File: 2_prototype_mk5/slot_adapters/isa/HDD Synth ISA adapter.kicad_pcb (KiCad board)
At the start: 2 copper layers, 119.4 x 97.4 mm, 16 parts, among them J1 Conn_01x02_Socket, J2 Conn_01x05_Socket, J3 Bus_ISA_8bit, J4 Conn_01x02_Socket, SW1 SW_Push, SW2 PEC12R-2120F-S0012

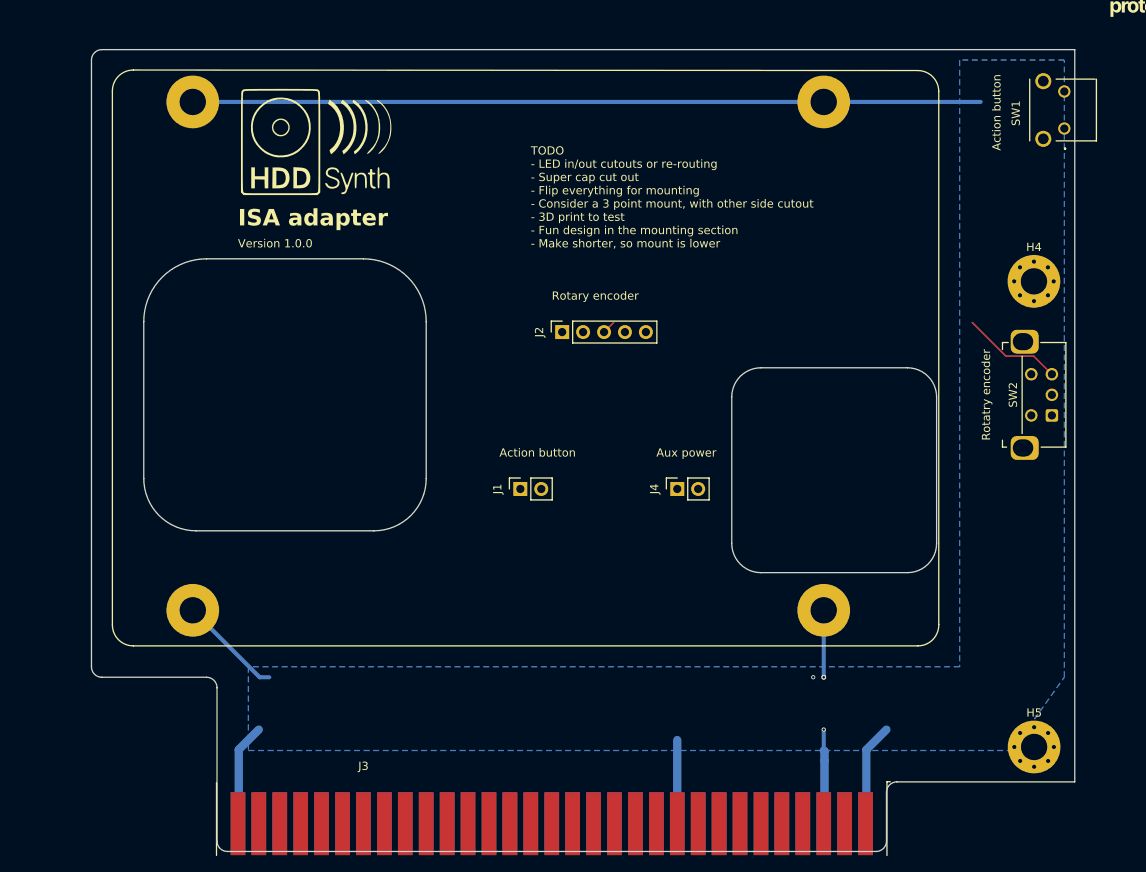
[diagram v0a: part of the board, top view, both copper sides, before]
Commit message: MK5 revision 2 hardware updates and ISA adapter revisions
Ignore VSCode local-history artifacts going forward.

Co-Authored-By: Claude Sonnet 5 <noreply@anthropic.com>
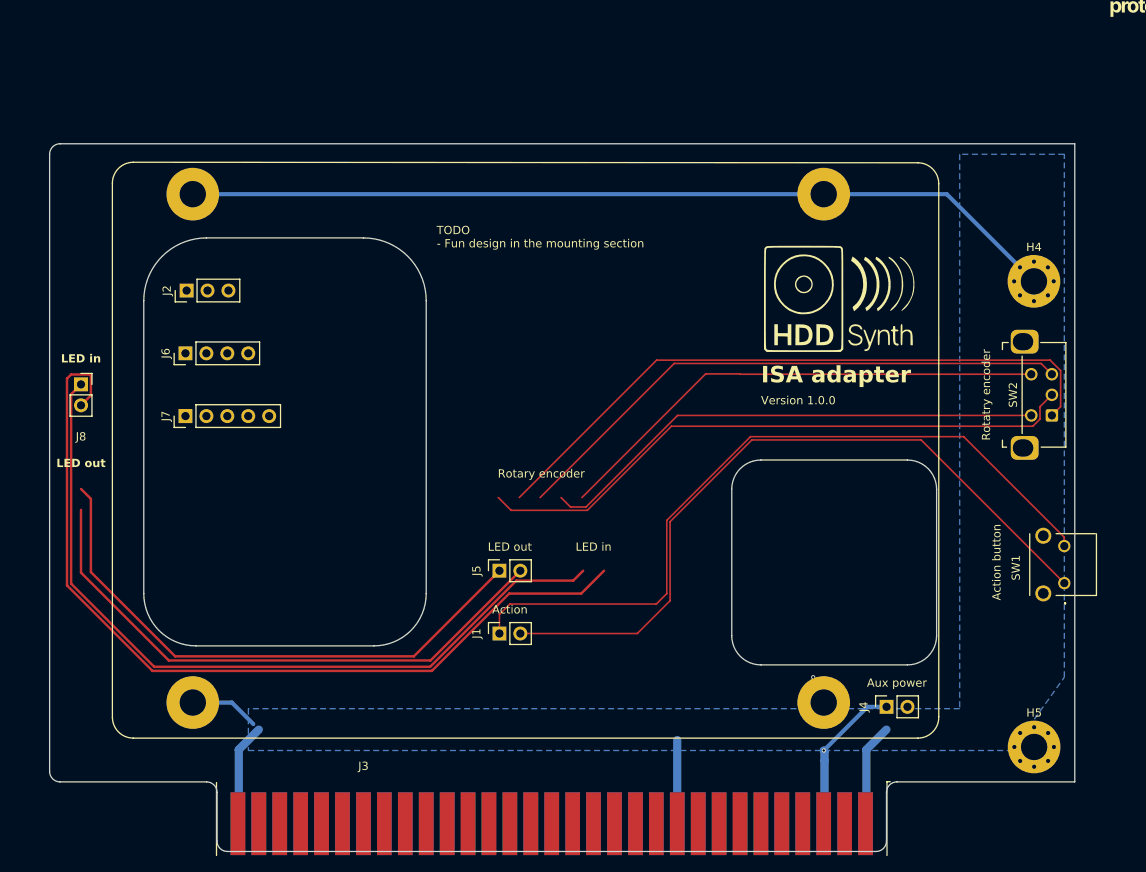
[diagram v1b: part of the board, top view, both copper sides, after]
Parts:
- removed  : LOGO, HDDSyncMKIII:MHDDLA_Sound_40mm
- added J5: Conn_01x02_Socket, Connector_PinSocket_2.54mm:PinSocket_1x02_P2.54mm_Vertical, F.Cu at (158.6, 106.4)
- added J6: Conn_01x04_Pin, Connector_PinSocket_2.54mm:PinSocket_1x04_P2.54mm_Vertical, F.Cu at (120.5, 80.0)
- added J7: Conn_01x05, Connector_PinSocket_2.54mm:PinSocket_1x05_P2.54mm_Vertical, F.Cu at (120.5, 87.6)
- added J8: Conn_01x02_Socket, Connector_PinSocket_2.54mm:PinSocket_1x02_P2.54mm_Vertical, F.Cu at (107.8, 83.8)
- J2: value Conn_01x05_Socket -> Conn_01x03; footprint Connector_PinSocket_2.54mm:PinSocket_1x05_P2.54mm_Vertical -> Connector_PinSocket_2.54mm:PinSocket_1x03_P2.54mm_Vertical
- moved G*** 66.3 mm to (200.5, 73.6)
- moved SW1 55.2 mm to (227.2, 107.9)
- moved J2 45.9 mm to (120.7, 72.4)
- moved G*** 36.9 mm to (198.0, 77.4)
- moved J4 36.7 mm to (205.6, 122.9)
- moved J1 17.7 mm to (158.6, 114.0)
- moved H11 11.2 mm to (198.0, 122.4)
- moved H9 11.2 mm to (121.4, 122.4)
- moved H10 11.2 mm to (198.0, 60.7)
- moved H8 11.2 mm to (121.4, 60.7)
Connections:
- J2 pad 1: Net-(J2-Pin_1) -> /RP2350/SWCLK
- J2 pad 2: /ENC_A -> GND
- J2 pad 3: /ENC_B -> /RP2350/SWD
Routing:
- net Net-(J7-Pin_2): track 0.00 -> 107.0 mm
- net Net-(J7-Pin_1): track 0.00 -> 95.9 mm
- net Net-(J1-Pin_1): track 0.00 -> 91.2 mm
- net Net-(J1-Pin_2): track 0.00 -> 88.6 mm
- net /ENC_A: track 0.00 -> 79.0 mm
- net Net-(J2-Pin_1): track 0.00 -> 74.5 mm
- net Net-(J5-Pin_2): track 0.00 -> 69.9 mm
- net Net-(J5-Pin_1): track 0.00 -> 68.7 mm
- net /ENC_SWITCH: track 0.00 -> 62.2 mm
- net Net-(J2-Pin_5): track 0.00 -> 60.8 mm
- net /ENC_B: track 13.9 -> 69.4 mm
- net Net-(J4-Pin_1): track 12.3 -> 18.4 mm
- net GND: track 128.2 -> 126.7 mm, vias 2 -> 1
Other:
- board size 119.4 x 97.4 mm -> 124.5 x 85.9 mm
- board text added: "Action"
- board text added: "LED in"
- board text added: "LED out"
- board text added: "TODO - Fun design in the mounting section"
- board text removed: "TODO - LED in/out cutouts or re-routing - Super cap cut out - Flip everything for mounting - Consider a 3 point mount, with other side cutout - 3D print to test - Fun design in the mounting section - Make shorter, so mount is lower"
